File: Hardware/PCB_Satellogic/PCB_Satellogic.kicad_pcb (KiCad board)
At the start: 2 copper layers, 92.7 x 78.7 mm, 4 parts, among them U1 E22-900M30S_LoRa, U2 Node-MCU_ESP32_38PINES, U3 TP4065_Modulo_cargador_de_bat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

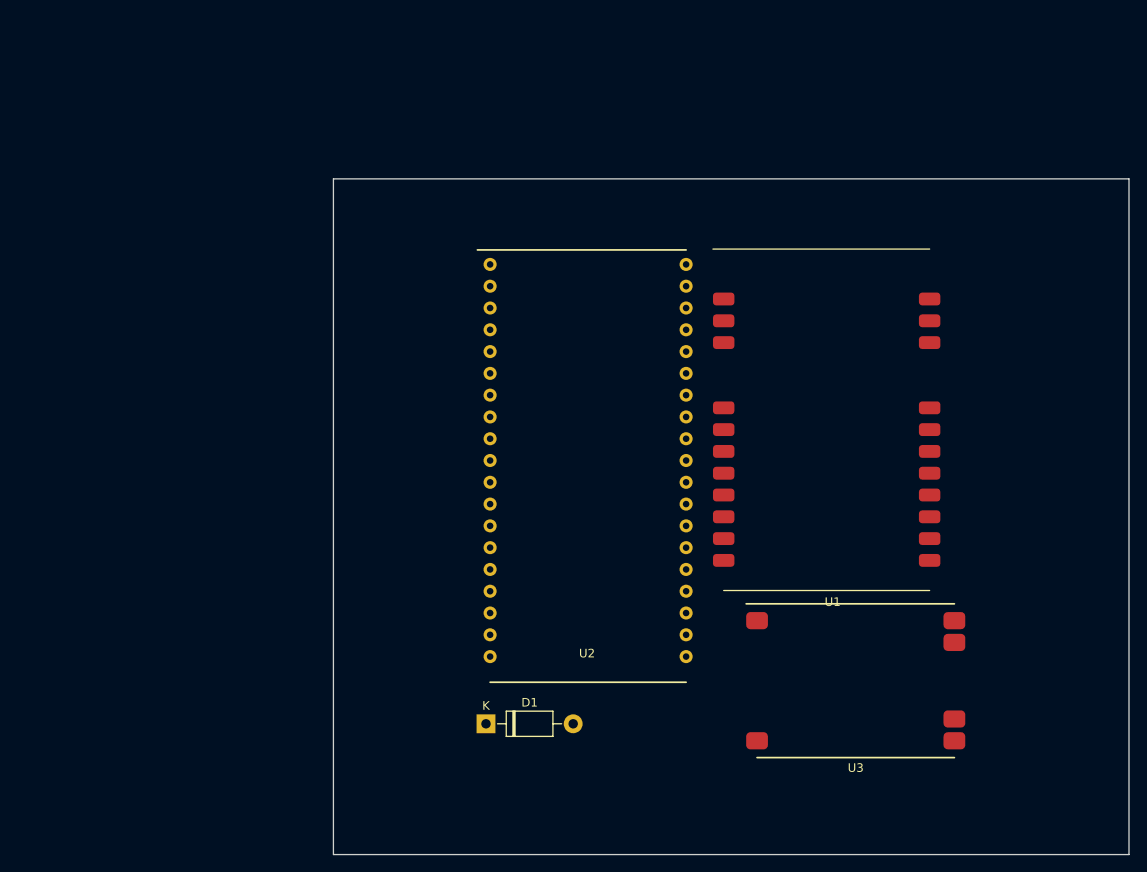
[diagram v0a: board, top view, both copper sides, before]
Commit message: Introducción HW
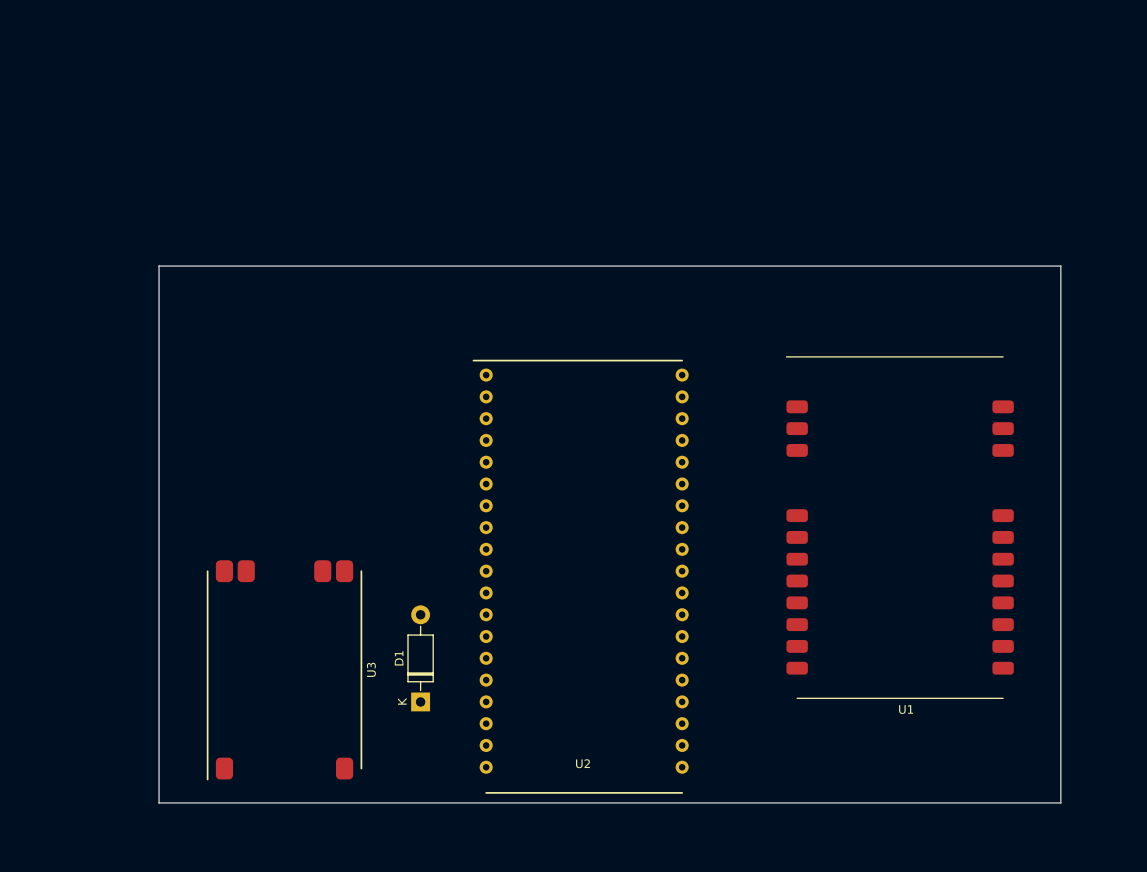
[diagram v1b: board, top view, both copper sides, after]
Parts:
- moved U3 66.6 mm to (98.4, 146.1), turned to 90 degrees
- moved U1 15.2 mm to (170.2, 129.5)
- moved U2 12.9 mm to (133.4, 134.6)
- moved D1 8.03 mm to (114.3, 149.9), turned to 90 degrees
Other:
- board size 92.7 x 78.7 mm -> 105.1 x 62.6 mm

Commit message: Introducción HW
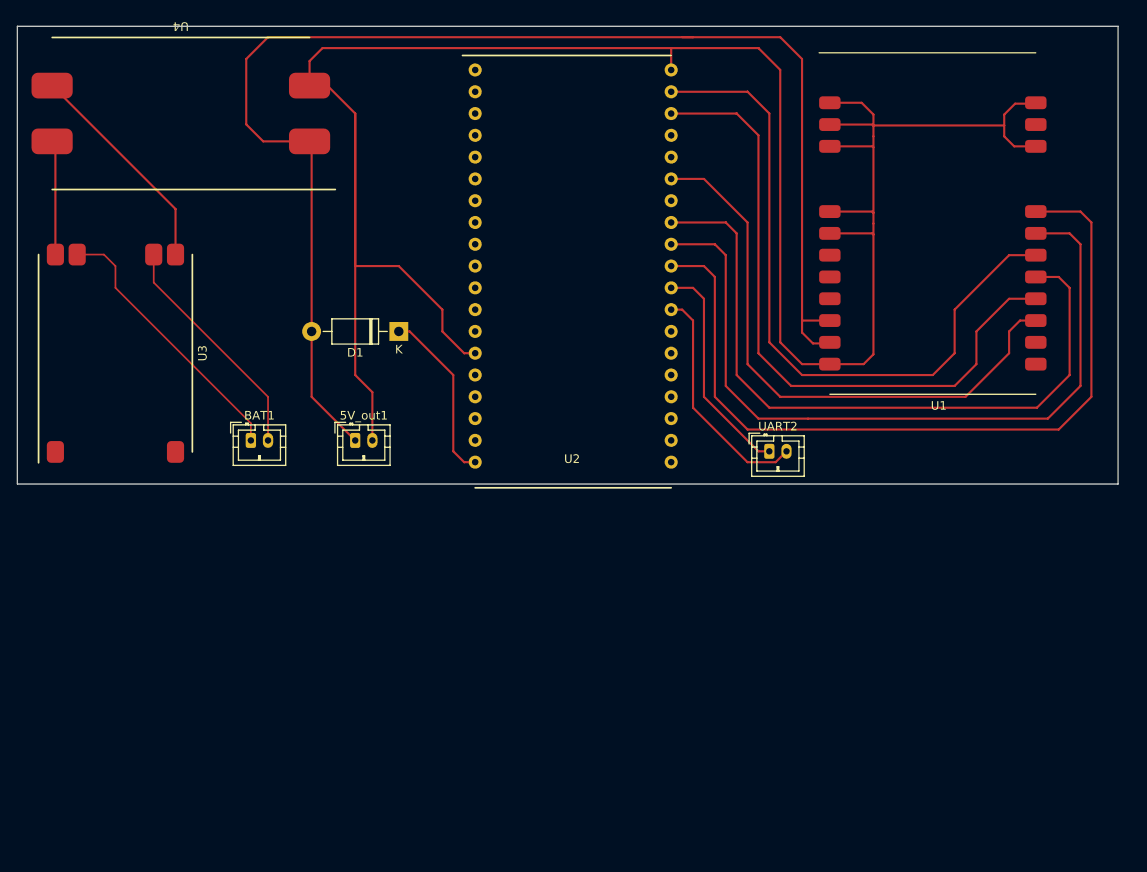
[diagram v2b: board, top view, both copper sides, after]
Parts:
- added 5V_out1: Conn_01x02, Connector_JST:JST_PH_B2B-PH-K_1x02_P2.00mm_Vertical, F.Cu at (106.7, 119.4)
- added BAT1: Conn_01x02, Connector_JST:JST_PH_B2B-PH-K_1x02_P2.00mm_Vertical, F.Cu at (94.5, 119.4)
- added U4: MT3608-Convertidor_Boost, PCB_Satellogic:MT3608-Convertidor_Boost, F.Cu at (86.4, 81.3)
- added UART2: Conn_01x02, Connector_JST:JST_PH_B2B-PH-K_1x02_P2.00mm_Vertical, F.Cu at (154.9, 120.7)
- U3: footprint PCB_Satellogic:TP4056 -> PCB_Satellogic:TP4056 - Módulo de carga de batería
- moved D1 43.3 mm to (111.8, 106.7), turned to 180 degrees
- moved U3 41.8 mm to (78.7, 109.2)
- moved U1 35.6 mm to (174.0, 94.1)
- moved U2 35.6 mm to (132.1, 99.1)
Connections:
- D1 pad 1: unconnected-(D1-K-Pad1) -> Net-(D1-K)
- D1 pad 2: unconnected-(D1-A-Pad2) -> /5V
- U1 pad 1: unconnected-(U1-GND-Pad1) -> /GND
- U1 pad 10: unconnected-(U1-Vcc-Pad10) -> /5V
- U1 pad 11: unconnected-(U1-GND-Pad11) -> /GND
- U1 pad 12: unconnected-(U1-GND-Pad12) -> /GND
- U1 pad 14: unconnected-(U1-BUSY-Pad14) -> /BUSY
- U1 pad 15: unconnected-(U1-NRST-Pad15) -> /RST_E22
- U1 pad 16: unconnected-(U1-MISO-Pad16) -> /MISO
- U1 pad 17: unconnected-(U1-MOSI-Pad17) -> /MOSI
- U1 pad 18: unconnected-(U1-SCK-Pad18) -> /SCK
- U1 pad 19: unconnected-(U1-NSS-Pad19) -> /NSS
- U1 pad 2: unconnected-(U1-GND-Pad2) -> /GND
- U1 pad 20: unconnected-(U1-GND-Pad20) -> /GND
- U1 pad 22: unconnected-(U1-GND-Pad22) -> /GND
- U1 pad 3: unconnected-(U1-GND-Pad3) -> /GND
- U1 pad 4: unconnected-(U1-GND-Pad4) -> /GND
- U1 pad 5: unconnected-(U1-GND-Pad5) -> /GND
- U1 pad 6: unconnected-(U1-RXEN-Pad6) -> /RXEN
- U1 pad 7: unconnected-(U1-TXEN-Pad7) -> /TXEN
- U1 pad 9: unconnected-(U1-Vcc-Pad9) -> /5V
- U2 pad 14: unconnected-(U2-GND-Pad14) -> /GND
- U2 pad 19: unconnected-(U2-Vin-Pad19) -> Net-(D1-K)
- U2 pad 27: unconnected-(U2-GPIO16-Pad27) -> /Rx2
- U2 pad 28: unconnected-(U2-GPIO17-Pad28) -> /Tx2
- U2 pad 29: unconnected-(U2-GPIO5-Pad29) -> /NSS
- U2 pad 30: unconnected-(U2-GPIO18-Pad30) -> /SCK
- U2 pad 31: unconnected-(U2-GPIO19-Pad31) -> /MISO
- U2 pad 33: unconnected-(U2-GPIO21-Pad33) -> /BUSY
- U2 pad 36: unconnected-(U2-GPIO22-Pad36) -> /RST_E22
- U2 pad 37: unconnected-(U2-GPIO23-Pad37) -> /MOSI
- U2 pad 38: unconnected-(U2-GND-Pad38) -> /GND
- U3 pad 3: unconnected-(U3-OUT--Pad3) -> Net-(U3-OUT-)
- U3 pad 4: unconnected-(U3-BAT--Pad4) -> /BAT-
- U3 pad 5: unconnected-(U3-BAT+-Pad5) -> /BAT+
- U3 pad 6: unconnected-(U3-OUT+-Pad6) -> Net-(U3-OUT+)
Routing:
- net /GND: track 0.00 -> 270.3 mm
- net /5V: track 0.00 -> 161.0 mm
- net /NSS: track 0.00 -> 93.9 mm
- net /SCK: track 0.00 -> 88.9 mm
- net /MISO: track 0.00 -> 81.3 mm
- net /MOSI: track 0.00 -> 80.6 mm
- net /RST_E22: track 0.00 -> 77.0 mm
- net /BUSY: track 0.00 -> 67.9 mm
- net /BAT+: track 0.00 -> 31.9 mm
- net /Rx2: track 0.00 -> 27.3 mm
- net /BAT-: track 0.00 -> 27.2 mm
- net /Tx2: track 0.00 -> 26.0 mm
- net Net-(U3-OUT-): track 0.00 -> 25.6 mm
- net Net-(D1-K): track 0.00 -> 20.4 mm
- net Net-(U3-OUT+): track 0.00 -> 13.3 mm
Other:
- board size 105.1 x 62.6 mm -> 128.3 x 53.3 mm
